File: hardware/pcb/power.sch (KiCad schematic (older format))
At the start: 18 parts, among them CON1 USB-MICRO-B, J2 LiPoly_Conn, U7 BQ24040DSQ, U8 TPS783

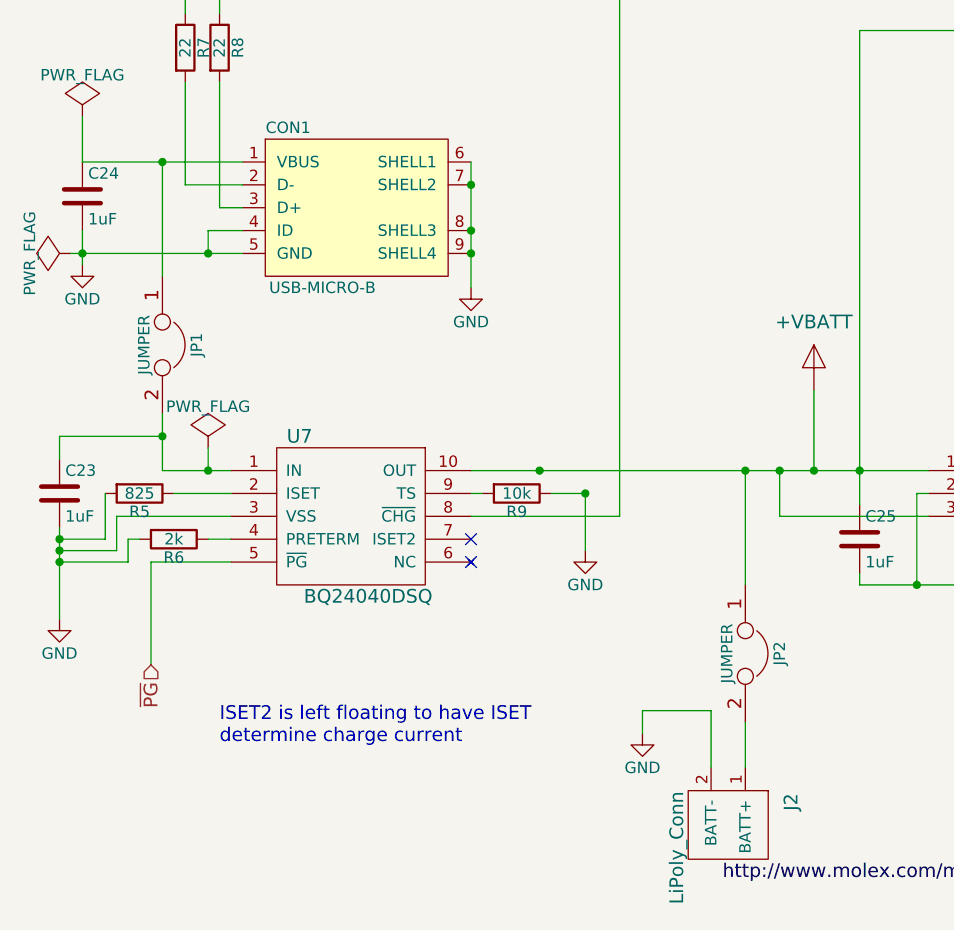
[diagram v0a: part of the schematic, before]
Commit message: pre-net import
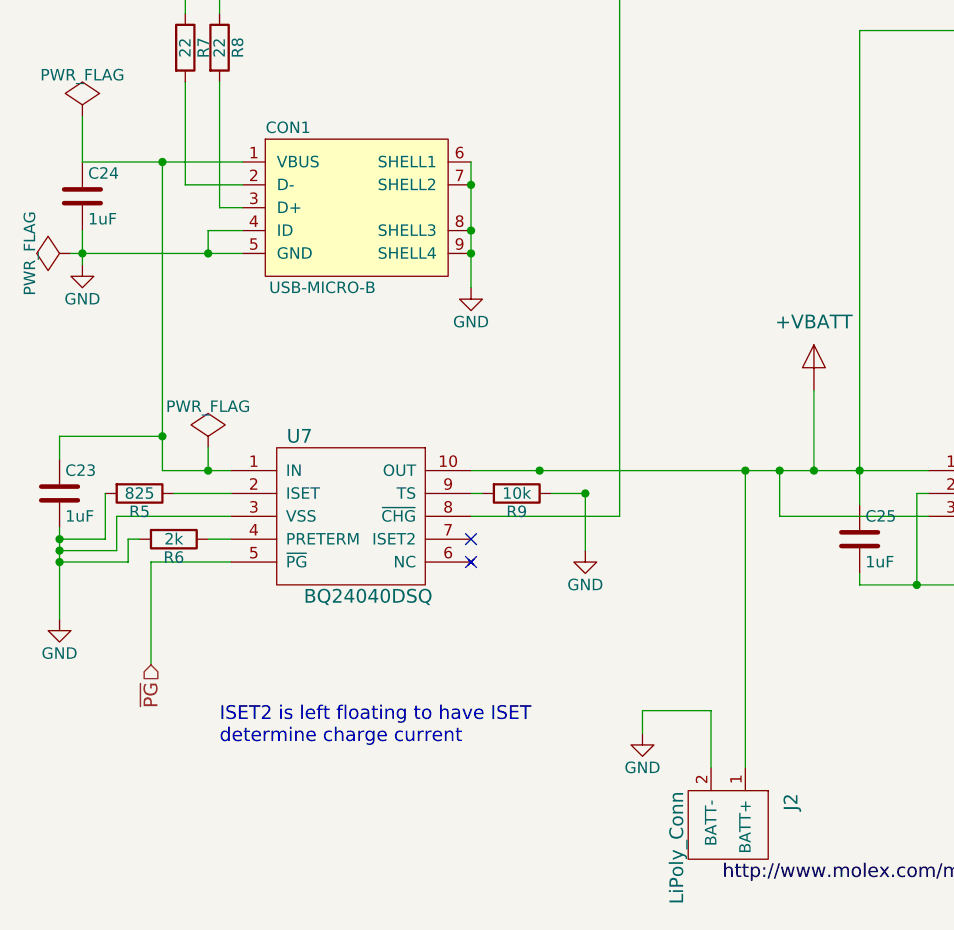
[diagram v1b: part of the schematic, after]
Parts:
- removed JP1, JP2: JUMPER, aero:Pin_Header_1x02_2mm, symbol JUMPER
- J2: footprint aero:Conn_Molex_78171-02 -> Pin_Headers:Pin_Header_Straight_1x02
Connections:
- net Vbatt: now also J2.1 (BATT+)
- net at C24.1, CON1.1 (VBUS): now also C23.1, U7.1 (IN)
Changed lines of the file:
@@
 F 0 "J2" H 5000 5900 60  0000 C CNN
 F 1 "LiPoly_Conn" H 5200 5400 60  0000 C CNN
-F 2 "aero:Conn_Molex_78171-02" H 5050 5500 60  0001 C CNN
+F 2 "Pin_Headers:Pin_Header_Straight_1x02" H 5050 5500 60  0001 C CNN
 F 3 "" H 5050 5500 60  0000 C CNN
 	1    5050 5500
@@
 	1    0    0    -1
 $EndComp
-$Comp
-L JUMPER JP1
-U 1 1 5540E544
-P 2700 3450
-F 0 "JP1" H 2700 3600 50  0000 C CNN
-F 1 "JUMPER" H 2700 3370 50  0000 C CNN
-F 2 "aero:Pin_Header_1x02_2mm" H 2700 3450 60  0001 C CNN
-F 3 "" H 2700 3450 60  0000 C CNN
-	1    2700 3450
-	0    1    1    0
-$EndComp
-$Comp
-L JUMPER JP2
-U 1 1 5540E5FA
-P 5250 4800
-F 0 "JP2" H 5250 4950 50  0000 C CNN
-F 1 "JUMPER" H 5250 4720 50  0000 C CNN
-F 2 "aero:Pin_Header_1x02_2mm" H 5250 4800 60  0001 C CNN
-F 3 "" H 5250 4800 60  0000 C CNN
-	1    5250 4800
-	0    1    1    0
-$EndComp
 Wire Wire Line
-	2700 3750 2700 4000
+	2700 2650 2700 4000
 Wire Wire Line
-	2700 3150 2700 2650
-Wire Wire Line
-	5250 5100 5250 5300
+	5250 4000 5250 5300
 Wire Wire Line
 	2350 2450 2350 2650
@@
 Connection ~ 5250 4000
 Wire Wire Line
-	5250 4000 5250 4500
-Wire Wire Line
 	4800 5150 4800 5050
